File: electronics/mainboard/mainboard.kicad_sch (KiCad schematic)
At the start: 25 parts, among them Q1 TSM250N02CX_RFG, Q2 TSM250N02CX_RFG, SW1 SW_Push, SW10 SW_Push, SW11 SW_Push, SW12 SW_Push, SW13 SW_Push, SW14 SW_Push, SW15 SW_Push, SW2 SW_Push, SW3 SW_Push, SW4 SW_Push, SW5 SW_Push, SW6 SW_Push, SW7 SW_Push, SW8 SW_Push, SW9 SW_Push, U1 1022

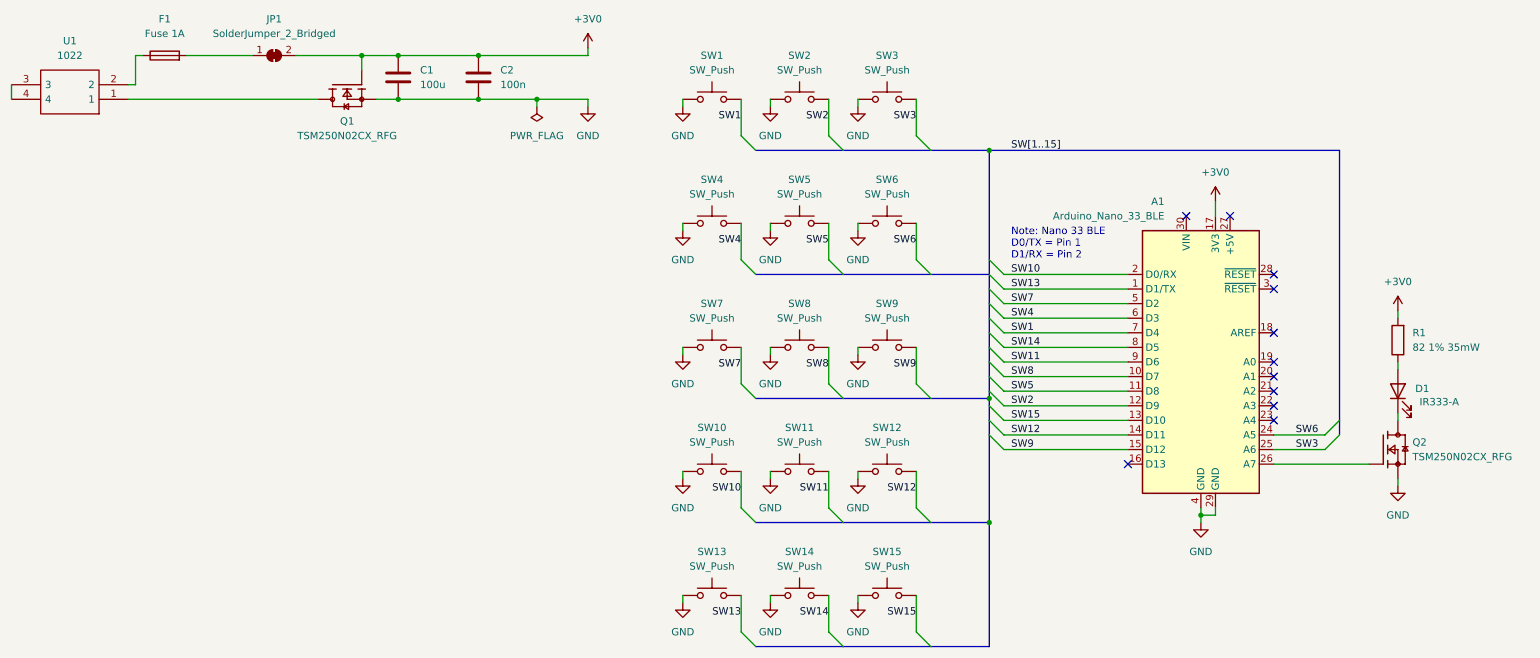
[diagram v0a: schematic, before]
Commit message: some changes
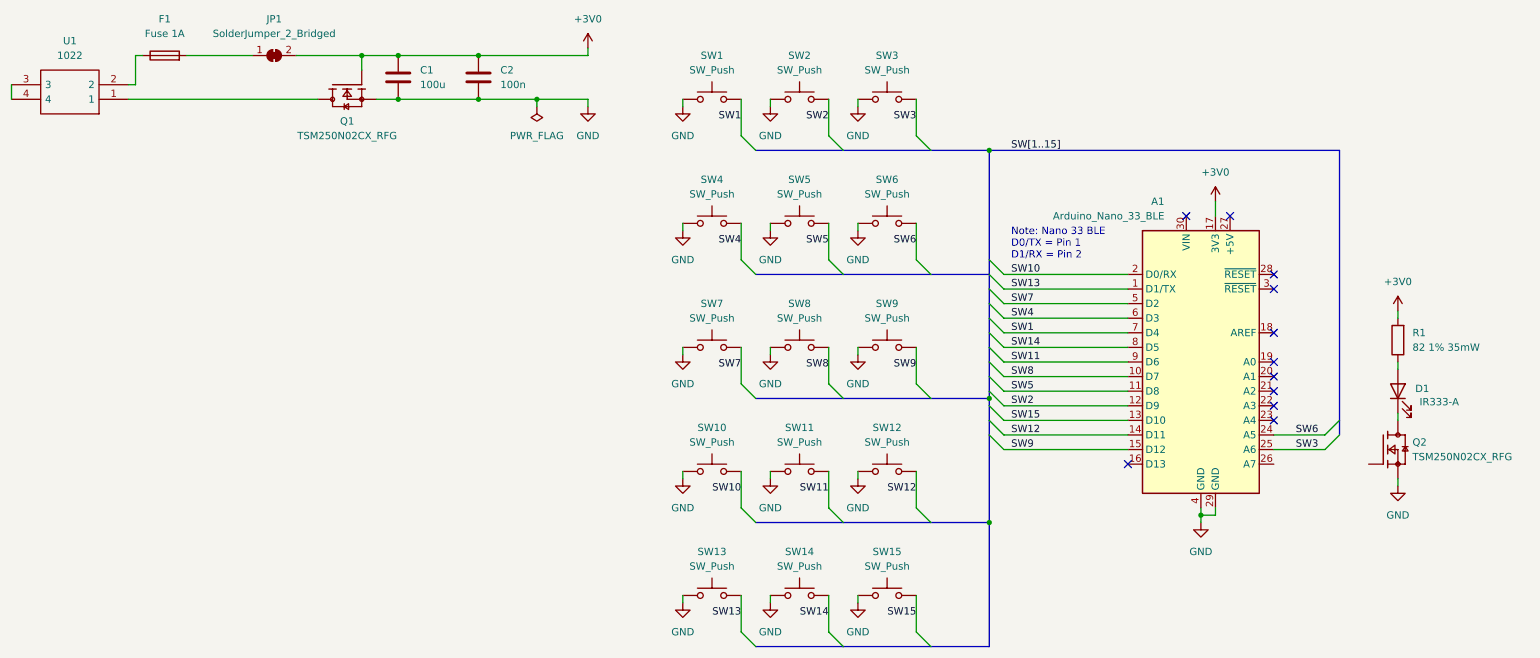
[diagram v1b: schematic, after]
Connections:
- net at A1.26 (A7): no longer Q2.1

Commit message: update symbols
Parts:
- Q1, Q2: footprint TSM250N02CX_RFG:TRANS_TSM250N02CX_RFG -> TRANS_TSM250N02CX_RFG
- U1: footprint SamacSys:1022 -> 1022
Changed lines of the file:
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@@
       (effects (font (size 1.27 1.27)))
     )
-    (property "Footprint" "TSM250N02CX_RFG:TRANS_TSM250N02CX_RFG" (at 73.66 45.72 0)
+    (property "Footprint" "TRANS_TSM250N02CX_RFG" (at 73.66 45.72 0)
       (effects (font (size 1.27 1.27)) (justify left bottom) hide)
     )
@@
       (effects (font (size 1.27 1.27)))
     )
-    (property "Footprint" "SamacSys:1022" (at 19.05 50.8 0)
+    (property "Footprint" "1022" (at 19.05 50.8 0)
       (effects (font (size 1.27 1.27)) (justify left) hide)
     )
@@
     )
   )
-  (symbol (lib_id "TSM250N02CX_RFG:TSM250N02CX_RFG") (at 254 109.22 0) (unit 1)
+  (symbol (lib_name "TSM250N02CX_RFG_1") (lib_id "TSM250N02CX_RFG:TSM250N02CX_RFG") (at 254 109.22 0) (unit 1)
     (in_bom yes) (on_board yes) (dnp no) (fields_autoplaced)
     (property "Reference" "Q2" (at 259.08 107.9499 0)
@@
       (effects (font (size 1.27 1.27)) (justify left))
     )
-    (property "Footprint" "TSM250N02CX_RFG:TRANS_TSM250N02CX_RFG" (at 254 109.22 0)
+    (property "Footprint" "TRANS_TSM250N02CX_RFG" (at 254 109.22 0)
       (effects (font (size 1.27 1.27)) (justify left bottom) hide)
     )

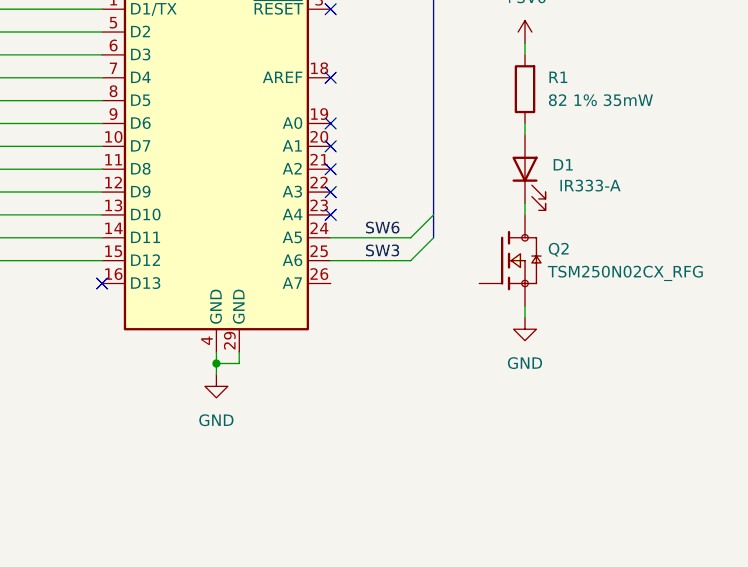
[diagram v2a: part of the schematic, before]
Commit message: error corrections
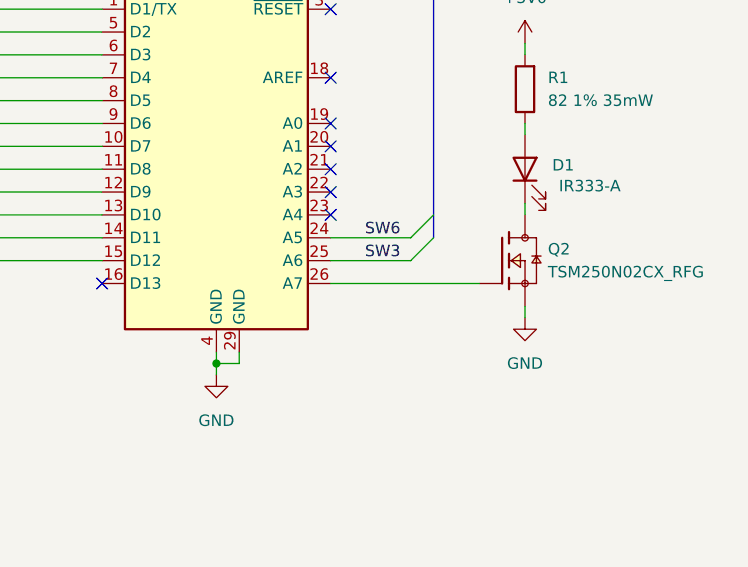
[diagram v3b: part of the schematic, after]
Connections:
- net at A1.26 (A7): now also Q2.1
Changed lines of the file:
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@@
+    (stroke (width 0) (type default))
+  )
+  (wire (pts (xy 234.95 111.76) (xy 251.46 111.76))
     (stroke (width 0) (type default))
   )
